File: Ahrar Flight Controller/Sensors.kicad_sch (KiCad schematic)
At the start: 7 parts, among them U3 MS5611-01BA

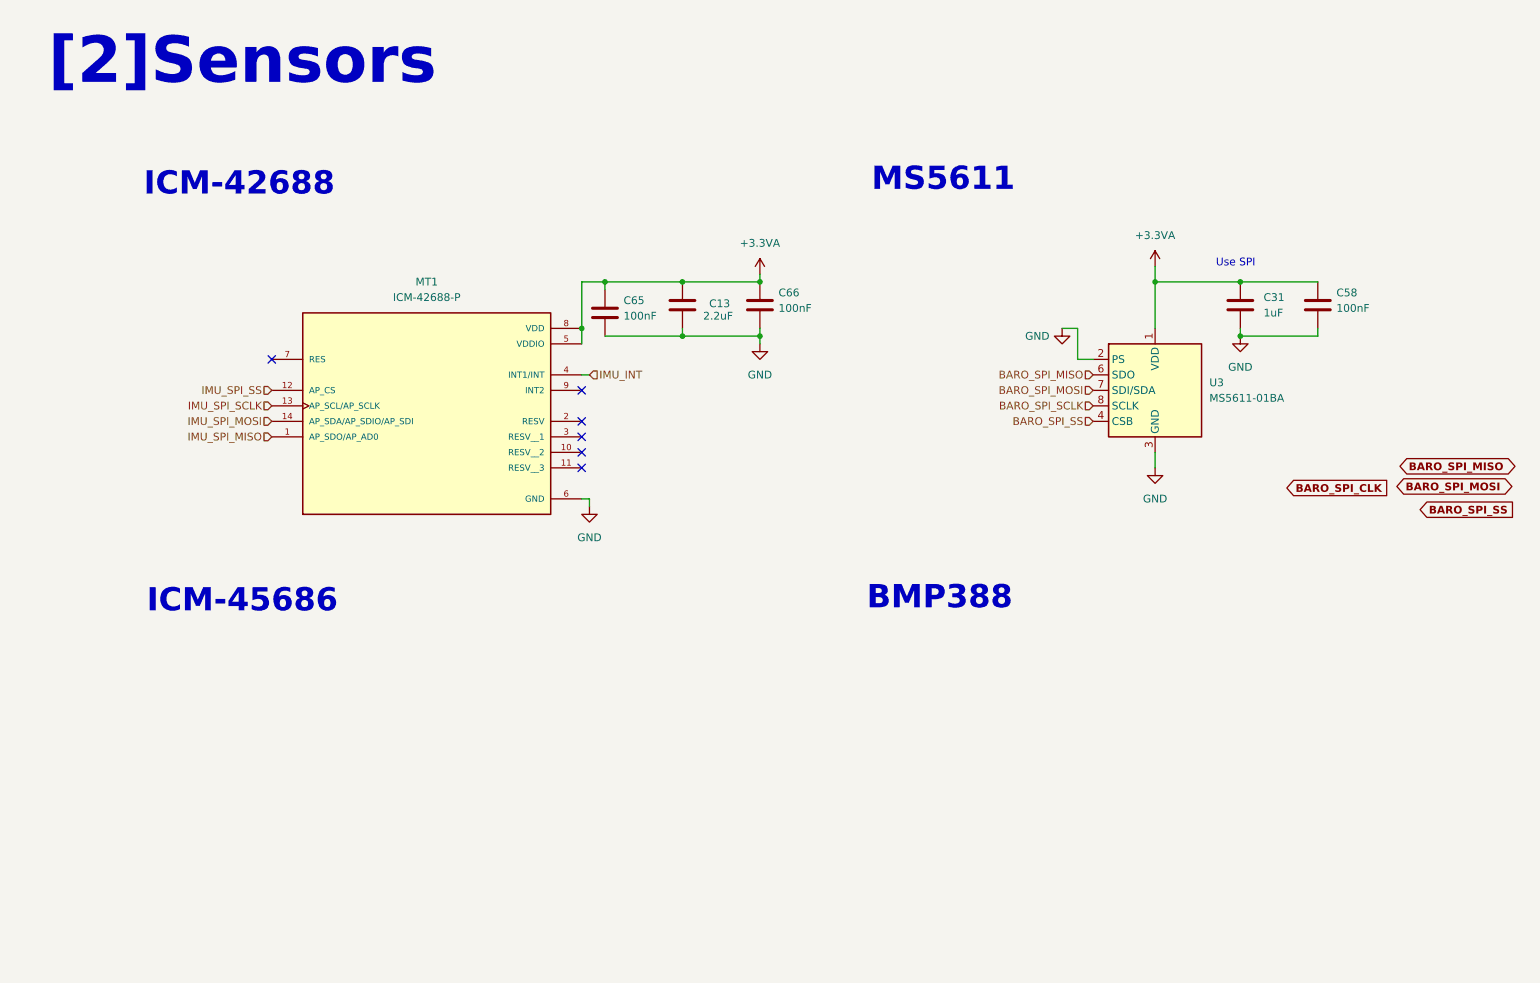
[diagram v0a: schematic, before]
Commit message: .
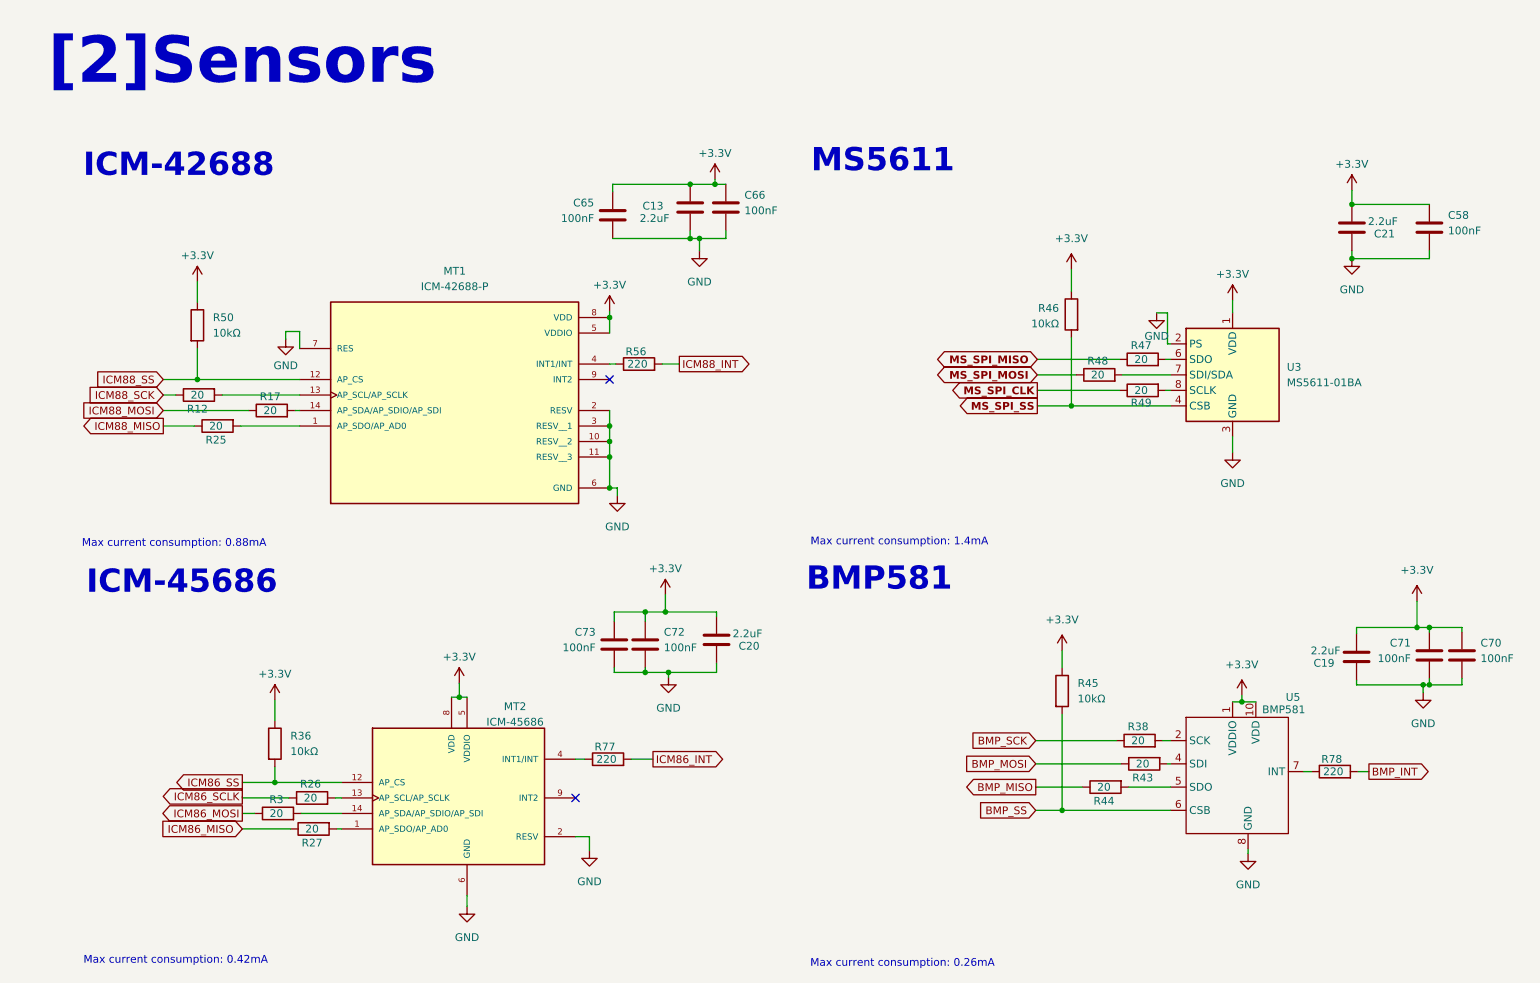
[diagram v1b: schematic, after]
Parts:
- removed C31: 1uF, Capacitor_SMD:C_0402_1005Metric, symbol Device:C
- added C19, C20, C21: 2.2uF, Capacitor_SMD:C_0603_1608Metric, symbol Device:C
- added C70, C71, C72, C73: 100nF, Capacitor_SMD:C_0402_1005Metric, symbol Device:C
- added MT2: ICM-45686, ICM_42688_P:LGA14_2P5X3X0P91_TDK-L, symbol ICM-42670-P:ICM-42670-P
- added R12, R17, R25, R26, R27, R3, R38, R43, R44, R47, R48, R49: 20, Resistor_SMD:R_0402_1005Metric, symbol Device:R
- added R36, R45, R46, R50: 10kΩ, Capacitor_SMD:C_0402_1005Metric, symbol Device:R
- added R56, R77, R78: 220, Resistor_SMD:R_0402_1005Metric, symbol Device:R
- added U5: BMP581, BMP581:BMP581, symbol IR2103STRPBF:BMP380
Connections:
- net GND: now also MT1.10 (RESV__2), MT1.11 (RESV__3), MT1.2 (RESV), MT1.3 (RESV__1), MT1.7 (RES), C19.2, C20.2, C21.2, C70.2, C71.2, C72.2, C73.2, MT2.10 (RESV__2), MT2.11 (RESV__3), MT2.2 (RESV), MT2.3 (RESV__1), MT2.6 (GND), MT2.7 (RESV), U5.3 (GND), U5.8 (GND), U5.9 (GND)
- net +3.3VA renamed +3.3V
- net +3.3V: now also C19.1, C20.1, C21.1, C70.1, C71.1, C72.1, C73.1, MT2.5 (VDDIO), MT2.8 (VDD), R36.1, R45.1, R46.1, R50.1, U5.1 (VDDIO), U5.10 (VDD)
- net BARO_SPI_MISO: no longer names the net of U3.6 (SDO)
- net BARO_SPI_MISO: now also R47.2
- net BARO_SPI_MOSI: no longer names the net of U3.7 (SDI/SDA)
- net BARO_SPI_MOSI: now also R48.2
- net BARO_SPI_SCLK: no longer names the net of U3.8 (SCLK)
- net BARO_SPI_SCLK: now also R49.2
- net BARO_SPI_SS renamed MS_SPI_SS
- net MS_SPI_SS: now also R46.2
- net IMU_INT: no longer names the net of MT1.4 (INT1/INT)
- net IMU_INT: now also R56.1
- net IMU_SPI_MISO: no longer names the net of MT1.1 (AP_SDO/AP_AD0)
- net IMU_SPI_MISO: now also R25.2
- net IMU_SPI_MOSI: no longer names the net of MT1.14 (AP_SDA/AP_SDIO/AP_SDI)
- net IMU_SPI_MOSI: now also R17.2
- net IMU_SPI_SCLK: no longer names the net of MT1.13 (AP_SCL/AP_SCLK)
- net IMU_SPI_SCLK: now also R12.2
- net IMU_SPI_SS renamed ICM88_SS
- net ICM88_SS: now also R50.2
- new net: R43.2, U5.4 (SDI)
- new net: MT2.13 (AP_SCL/AP_SCLK), R26.2
- new net: MT2.1 (AP_SDO/AP_AD0), R27.2
- new net: MT2.14 (AP_SDA/AP_SDIO/AP_SDI), R3.2
- new net: MT2.4 (INT1/INT), R77.1
- new net: R38.2, U5.2 (SCK)
- new net: R44.2, U5.5 (SDO)
- new net: R78.1, U5.7 (INT)
- new net BMP_INT: R78.2
- new net BMP_MISO: R44.1
- new net BMP_MOSI: R43.1
- new net BMP_SCK: R38.1
- new net BMP_SS: R45.2, U5.6 (CSB)
- new net ICM86_INT: R77.2
- new net ICM86_MISO: R27.1
- new net ICM86_MOSI: R3.1
- new net ICM86_SCLK: R26.1
- new net ICM86_SS: MT2.12 (AP_CS), R36.2
- new net ICM88_INT: R56.2
- new net ICM88_MISO: R25.1
- new net ICM88_MOSI: R17.1
- new net ICM88_SCK: R12.1
- new net MS_SPI_CLK: R49.1
- new net MS_SPI_MISO: R47.1
- new net MS_SPI_MOSI: R48.1
- no-connect marks 6 -> 2
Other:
- note added: "BMP581"
- note added: "Max current consumption: 0.26mA"
- note added: "Max current consumption: 0.42mA"
- note added: "Max current consumption: 0.88mA"
- note added: "Max current consumption: 1.4mA"
- note removed: "BMP388"
- note removed: "Use SPI"
- moved on the sheet: C13, C58, C65, C66, MT1, U3
